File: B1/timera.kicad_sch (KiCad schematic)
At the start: 15 parts, among them U108 74HC32, U109 74HC74, U110 74HC04, U113 74HC27, U114 74HC153, U115 74HC74, U118 74HC74, U119 74HC74, U121 74HC377, U122 74HC377, U123 74HCT74, U124 74HC00, U126 74HC00, U127 74HC08, U129 74HC74

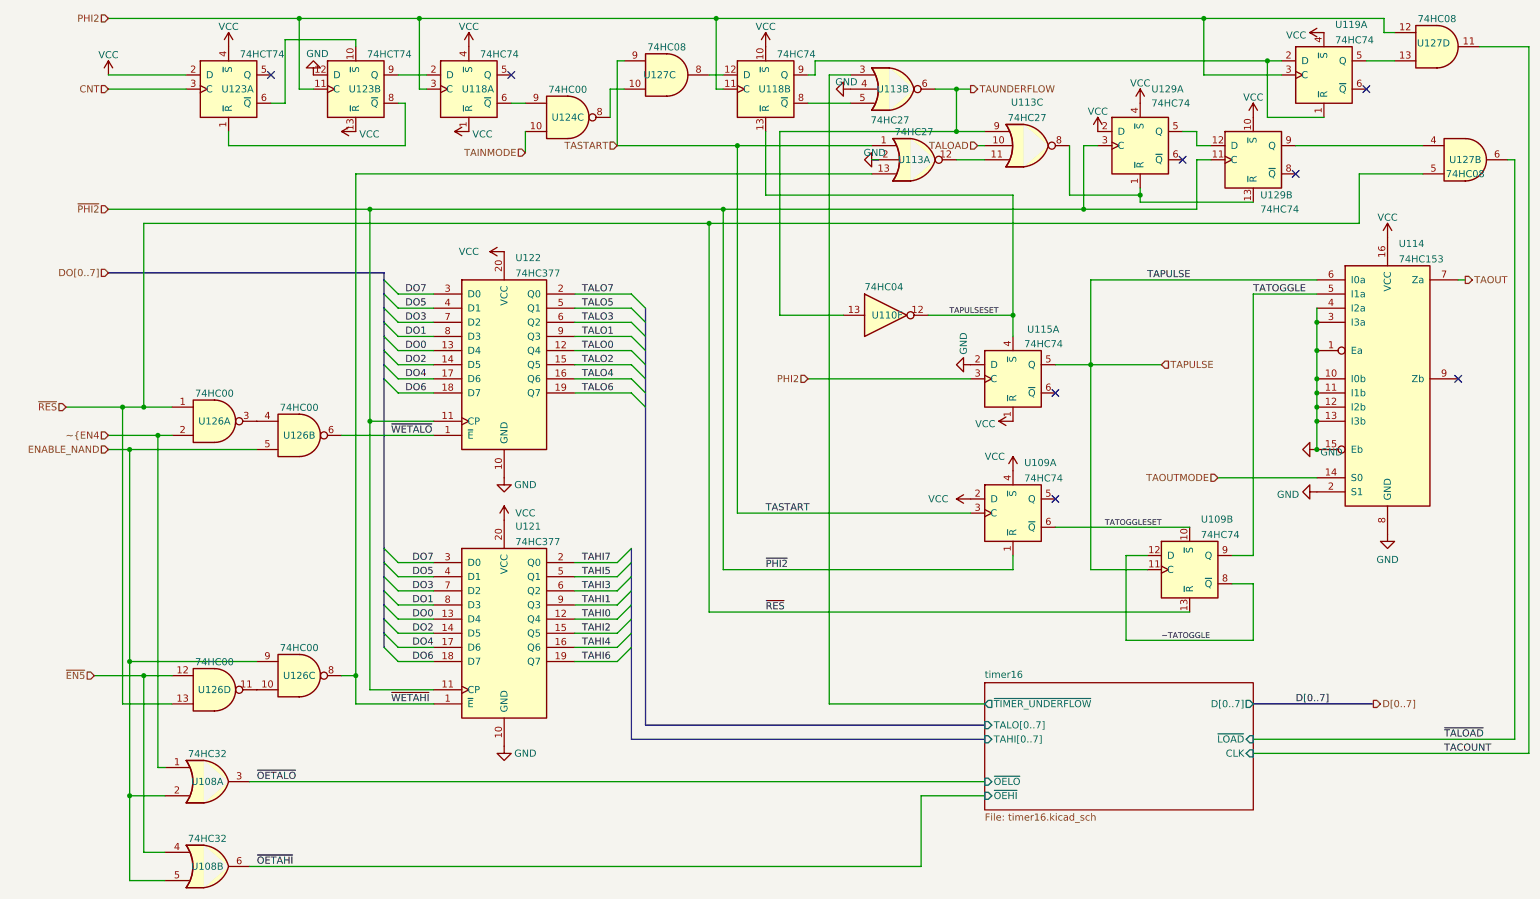
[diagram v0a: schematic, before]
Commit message: .
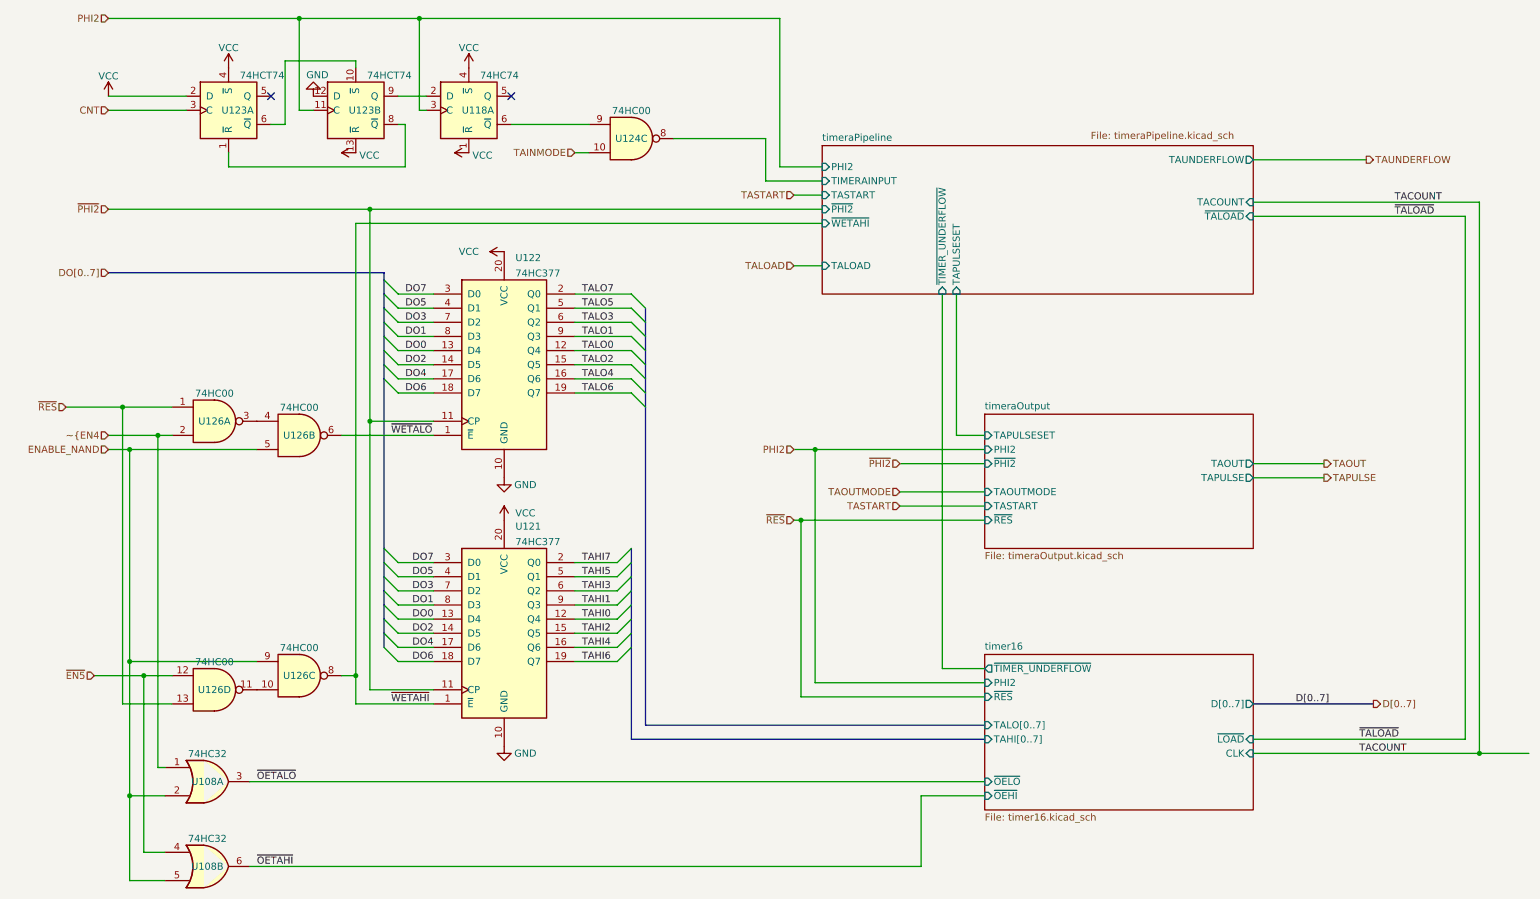
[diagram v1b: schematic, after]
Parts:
- removed U109, U115, U119, U129: 74HC74, Package_SO:SO-14_3.9x8.65mm_P1.27mm, symbol 74xx:74HC74
- removed U110: 74HC04, Package_SO:SOIC-14_3.9x8.7mm_P1.27mm, symbol 74xx:74HC04
- removed U113: 74HC27, Package_SO:SO-14_3.9x8.65mm_P1.27mm, symbol 74xx:74LS27
- removed U114: 74HC153, Package_SO:SOIC-16_3.9x9.9mm_P1.27mm, symbol 74xx:74LS153
- removed unit 2 of U118
- removed U127: 74HC08, Package_SO:SO-14_3.9x8.65mm_P1.27mm, symbol Custom 74xx:74HC08
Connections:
- net timeraPipeline/TIMERAINPUT: now reaches U124.8
- no-connect marks 8 -> 2
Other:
- added sheet timeraOutput (timeraOutput.kicad_sch)
- added sheet timeraPipeline (timeraPipeline.kicad_sch)
- sheet timer16 ports: added PHI2, ~{RES}; removed none
- moved on the sheet: U118A, U123A, U123B, U124C
